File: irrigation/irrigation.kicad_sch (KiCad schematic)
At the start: 47 parts, among them J1 24V Jmp, J10 24V, J11 25%, J12 50%, J13 75%, J14 100%, J15 100%, J16 100%, J17 Pump, J18 Outlet Pump, J2 Power, J20 25%, J21 25%, J22 PT 6-TWIN, J23 PT 6-TWIN, J3 Power, J4 Power, J5 Power, J6 Power, J7 Power, J8 0V Jmp, J9 Empty, K1 PLC-RPT-24DC/21, K2 PLC-RPT-24DC/21, K3 PLC-RPT-24DC/21, K4 PLC-RPT-24DC/21, M1 Well Pump, M2 Outlet Pump, SW1 Well Empty, SW2 100% Full, SW3 25% Full, SW4 50% Full, SW5 75% Full, SW6 Drain Switch, SW7 Fill Switch, U1 MPPT-Charger

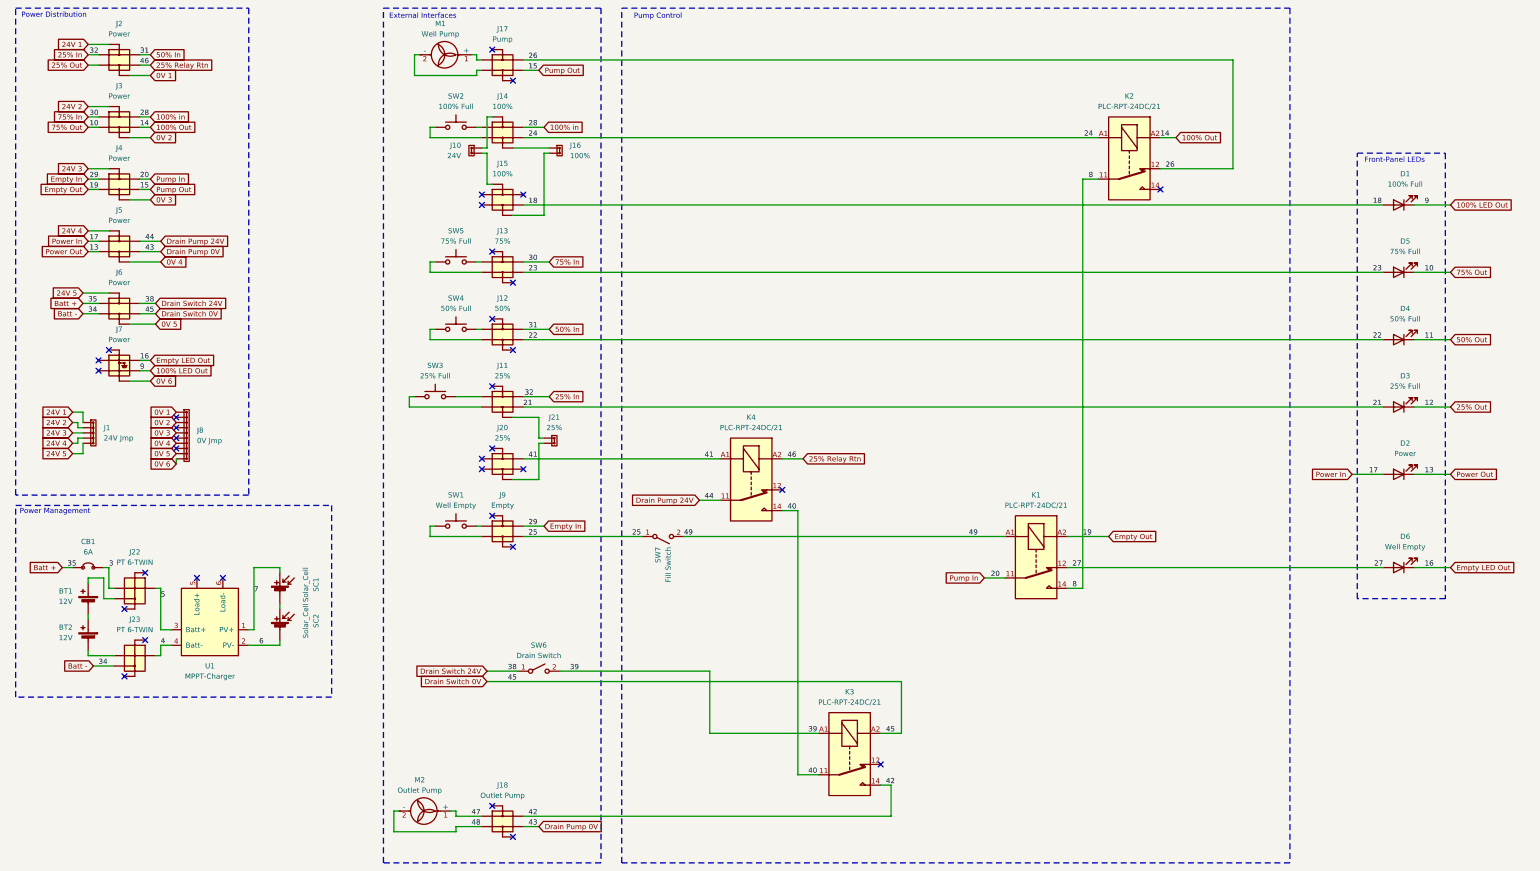
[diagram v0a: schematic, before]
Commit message: Cleanup for readme
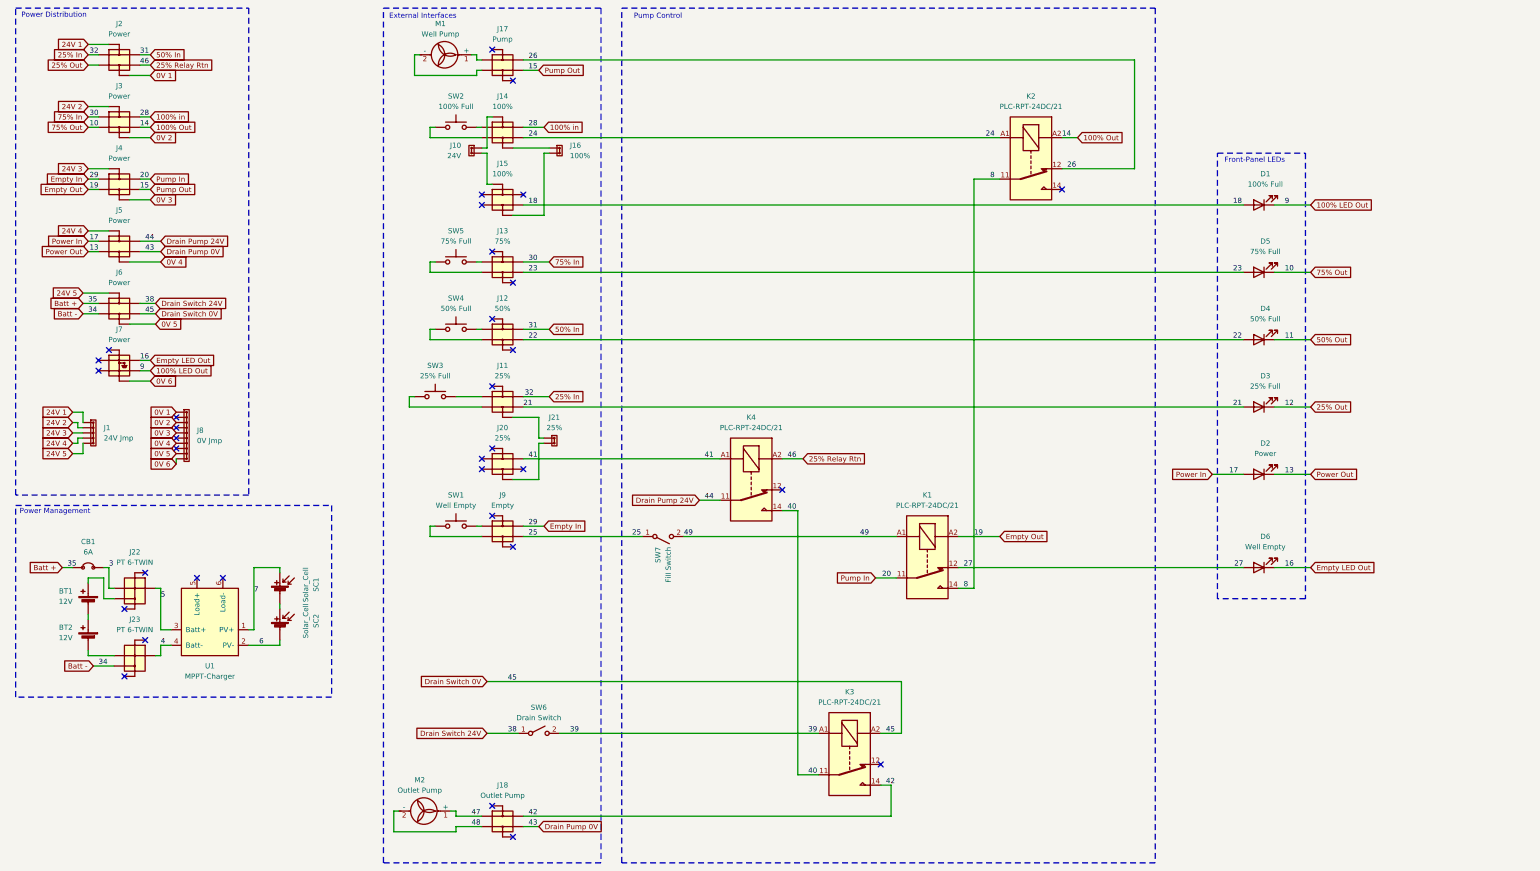
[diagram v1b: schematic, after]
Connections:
- net at J10.: now also J15.; no longer J14.
- net at J16.: now also J15.; no longer J14.
- net at J21.: now also J11.; no longer J20.
- new net: J10., J14.
- new net: J14., J16.
- new net: J20., J21.
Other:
- moved on the sheet: D1, D2, D3, D4, D5, D6, K1, K2, SW6
